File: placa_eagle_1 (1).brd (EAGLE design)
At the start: 88.2 x 35.5 mm, 19 parts, among them J1 CONN_0227-2021, J2 CONN_0427-2041, J3 CONN_0227-2021, J4 CONN_0227-2021, J5 CONN_0427-2041

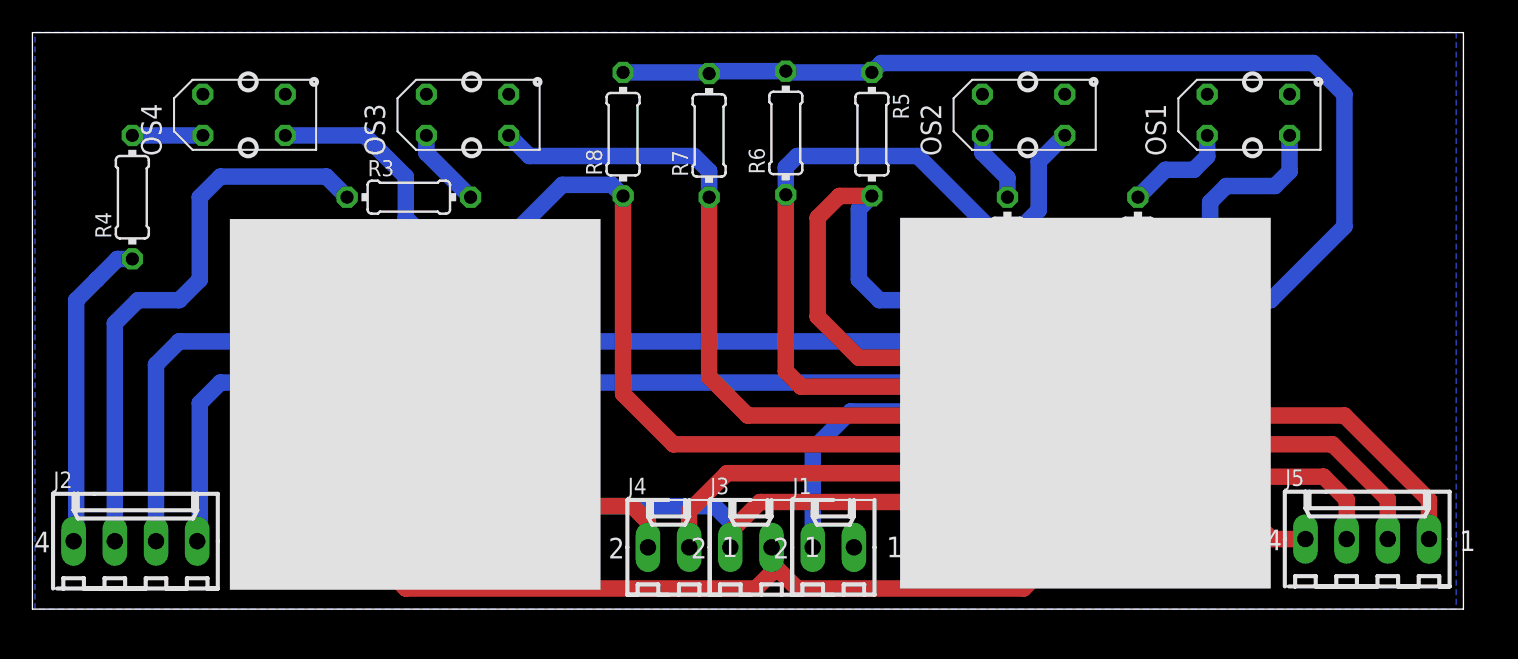
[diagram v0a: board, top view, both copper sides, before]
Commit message: Placa ataulizada.
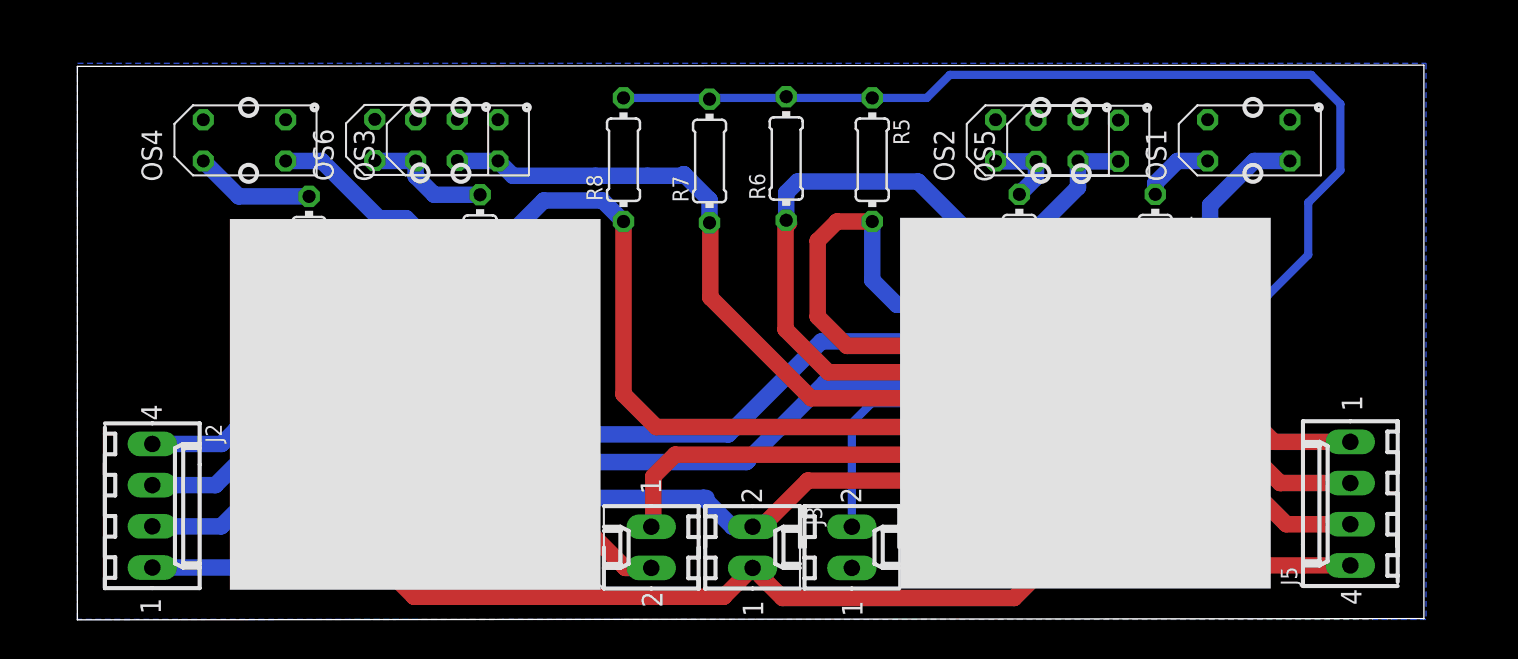
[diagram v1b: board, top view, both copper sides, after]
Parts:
- added OS5, OS6: (no value), Robotica-IFRN-SC-sensores:TCRT5000
- moved R4 11.5 mm to (19.4, 63.6)
- moved R3 5.72 mm to (30.0, 63.7), turned to 90 degrees
- moved J5 2.42 mm to (83.6, 48.4), turned to 90 degrees
- moved J2 2.42 mm to (9.77, 48.3), turned to 270 degrees
- moved OS2 1.77 mm to (64.3, 70.8)
- moved OS3 1.71 mm to (28.5, 70.8)
- moved R5 1.58 mm to (54.2, 69.6)
- moved R6 1.58 mm to (48.9, 69.7)
- moved R7 1.58 mm to (44.1, 69.5)
- moved R8 1.58 mm to (38.8, 69.6)
- moved OS1 1.58 mm to (77.4, 70.8)
- moved OS4 1.58 mm to (15.5, 70.8)
- moved J1 1.14 mm to (52.9, 45.7), turned to 270 degrees
- moved R1 1.08 mm to (71.6, 63.7)
- moved J4 1.07 mm to (40.5, 45.7), turned to 90 degrees
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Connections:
- removed net N$2: OS2.A, R2.2
- removed net N$3: OS3.A, R3.2
- removed net N$6: J5.2, OS2.C, R6.1
- removed net N$7: J5.3, OS3.C, R7.1
- new net N$15: OS2.A, OS5.A, R2.2
- new net N$17: J5.2, OS2.C, OS5.C, R6.1
- new net N$19: OS3.A, OS6.A, R3.2
- new net N$20: J5.3, OS3.C, OS6.C, R7.1
- net GND: now also OS5.E, OS5.K, OS6.E, OS6.K
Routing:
- net N$6: track 78.9 -> 0.00 mm
- net N$17: track 0.00 -> 72.2 mm
- net N$7: track 70.8 -> 0.00 mm
- net N$20: track 0.00 -> 67.9 mm
- net N$5: track 94.6 -> 79.8 mm
- net N$11: track 35.2 -> 26.8 mm
- net N$19: track 0.00 -> 7.91 mm
- net N$10: track 64.7 -> 58.8 mm
- net N$15: track 0.00 -> 4.96 mm
- net N$3: track 4.94 -> 0.00 mm
- net N$2: track 4.45 -> 0.00 mm
- net N$12: track 19.4 -> 16.1 mm
- net N$14: track 32.8 -> 36.2 mm
- net VCC: track 98.4 -> 95.2 mm
- net N$4: track 4.35 -> 7.43 mm
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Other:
- board size 88.2 x 35.5 mm -> 83 x 34.2 mm
